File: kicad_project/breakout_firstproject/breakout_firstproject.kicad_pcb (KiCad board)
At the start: 2 copper layers, 10 parts, among them J1 Conn_01x04_Male, J2 Conn_01x04_Male, U1 nrf24l01, U2 LM1117-3.3

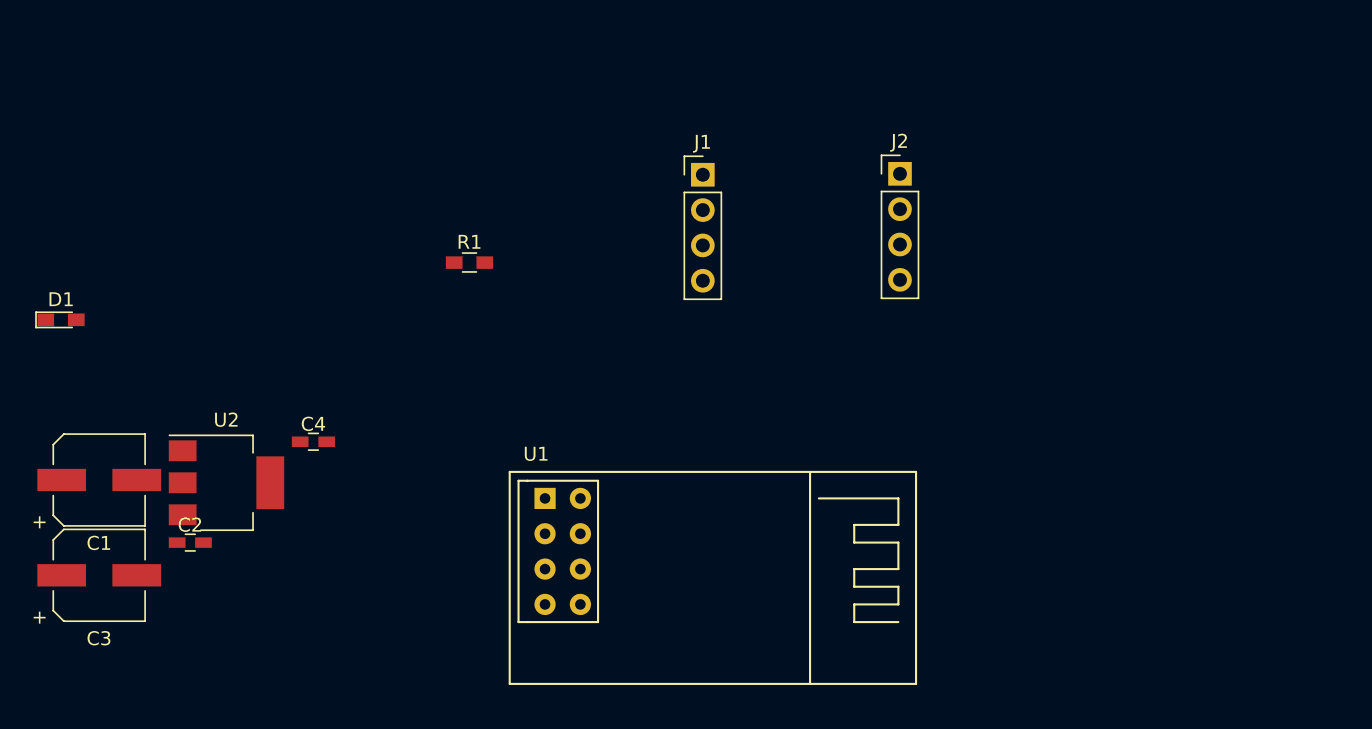
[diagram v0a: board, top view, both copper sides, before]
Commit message: added PCB final and gebers
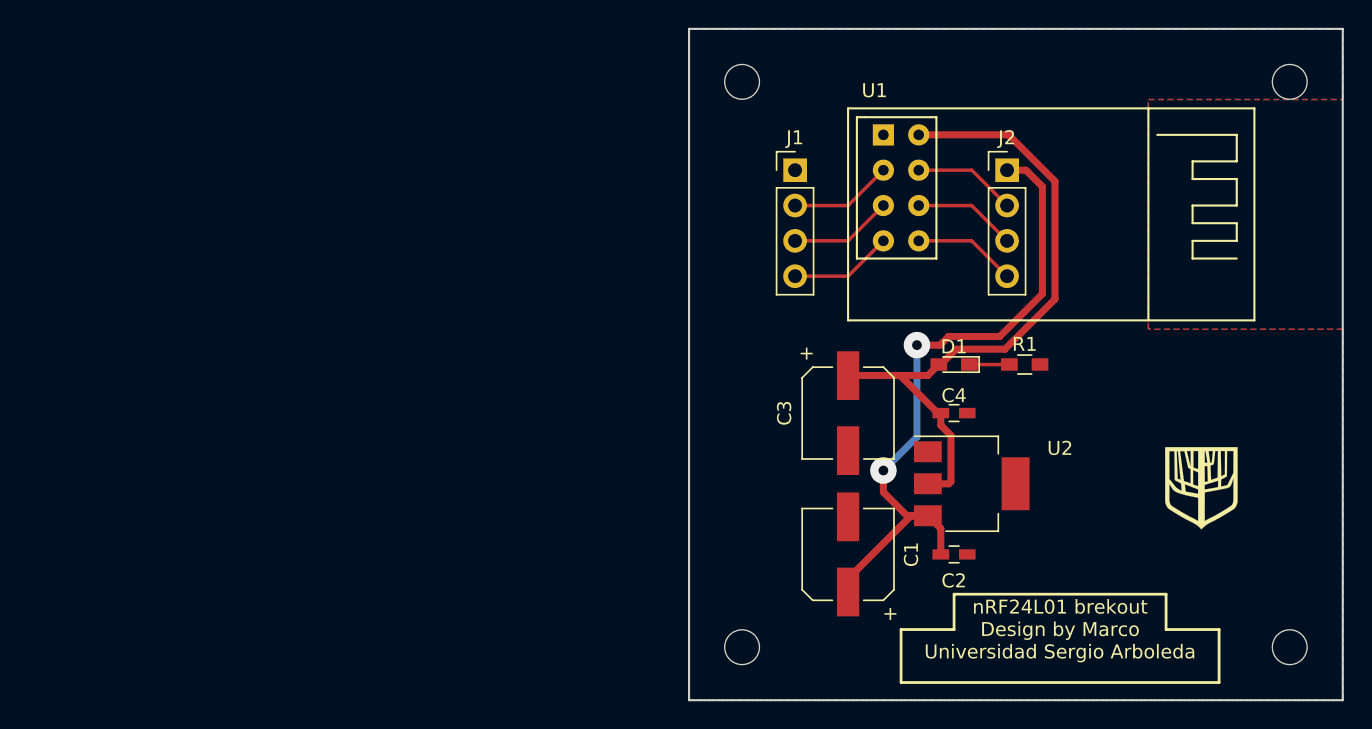
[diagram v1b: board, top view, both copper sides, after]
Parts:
- added G***: logousasmall, mycustomfootprints:logousasmall, F.Cu at (180.3, 97.8)
- added REF**: MountingHole_2.5mm, Mounting_Holes:MountingHole_2.5mm, F.Cu at (147.3, 109.2)
- added REF**: MountingHole_2.5mm, Mounting_Holes:MountingHole_2.5mm, F.Cu at (186.7, 109.2)
- added REF**: MountingHole_2.5mm, Mounting_Holes:MountingHole_2.5mm, F.Cu at (186.7, 68.6)
- added REF**: MountingHole_2.5mm, Mounting_Holes:MountingHole_2.5mm, F.Cu at (147.3, 68.6)
- moved D1 64.3 mm to (162.6, 88.9), turned to 180 degrees
- moved C3 55.1 mm to (154.9, 92.4), turned to 270 degrees
- moved C2 54.9 mm to (162.6, 102.5)
- moved C1 54.1 mm to (154.9, 102.5), turned to 90 degrees
- moved U2 53.6 mm to (163.8, 97.5)
- moved C4 46.1 mm to (162.6, 92.4)
- moved R1 40.6 mm to (167.6, 88.9)
- moved U1 35.7 mm to (162.6, 77.5)
- moved J2 7.70 mm to (166.4, 74.9)
- moved J1 6.64 mm to (151.1, 74.9)
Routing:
- net VCC: track 0.00 -> 48.5 mm, vias 0 -> 2
- net +3V3: track 0.00 -> 47.8 mm
- net SCK: track 0.00 -> 7.40 mm
- net MOSI: track 0.00 -> 7.40 mm
- net MISO: track 0.00 -> 7.40 mm
- net IRQ: track 0.00 -> 7.40 mm
- net CSN: track 0.00 -> 7.40 mm
- net CE: track 0.00 -> 7.40 mm
- net Net-(D1-Pad1): track 0.00 -> 2.88 mm
- added copper zone on B.Cu, net GND
- added copper zone on F.Cu, net GND
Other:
- board outline added: 47 x 48.3 mm
- net class Colcircuitos added: clearance 0.22, trace_width 0.25, via_dia 0.9, via_drill 0.4
- net class Power added: clearance 0.4, trace_width 0.508, via_dia 1.905, via_drill 0.7
- board text added: "Esto fue diseñado para la clase de Diseño de productos IoT"
- board text added: "No conectar luego de que caer un rayo"
- board text added: "nRF24L01 brekout Design by Marco Universidad Sergio Arboleda"
